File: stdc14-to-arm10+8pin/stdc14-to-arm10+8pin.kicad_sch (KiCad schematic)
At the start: 3 parts, among them J1 Conn_ARM_JTAG_SWD_10, J2 Conn_ST_STDC14, J3 Conn_02x04_Counter_Clockwise

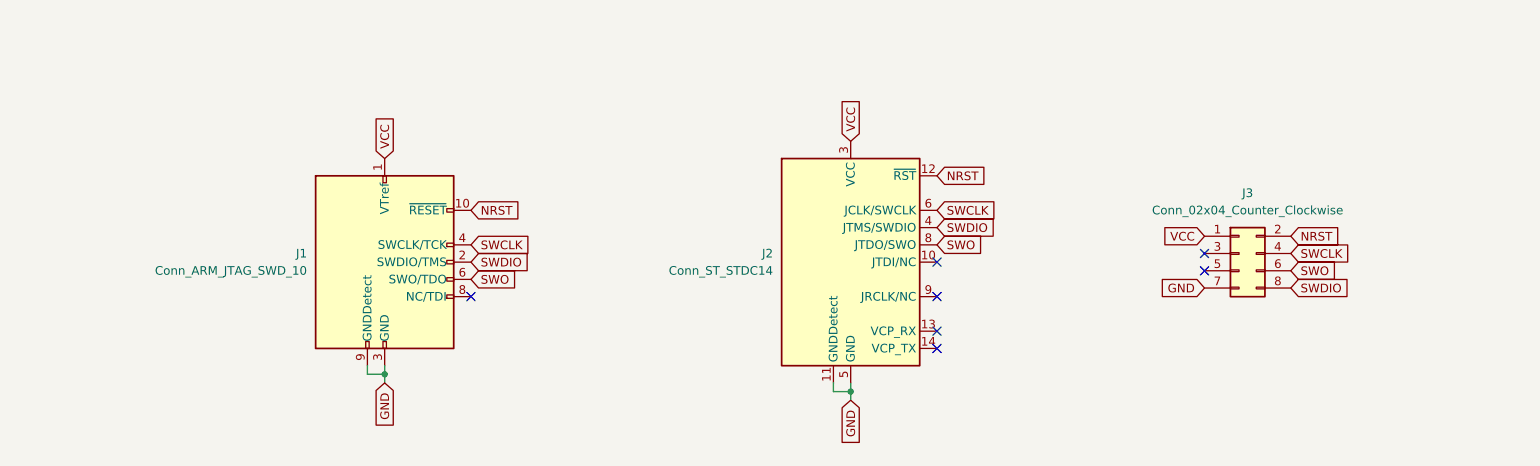
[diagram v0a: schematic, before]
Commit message: prob fin?
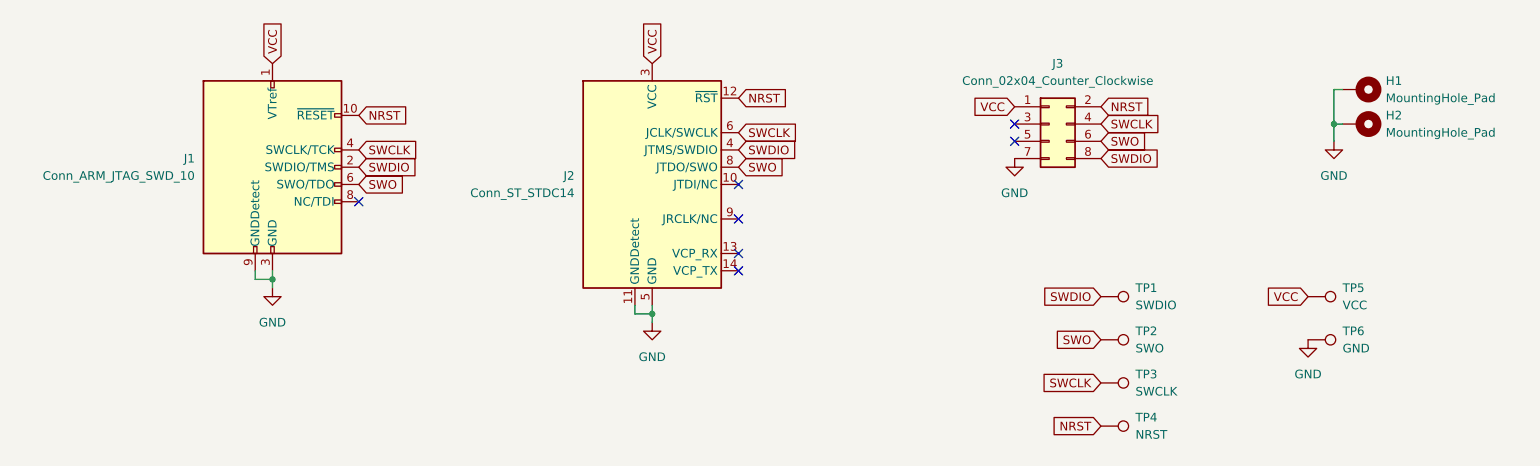
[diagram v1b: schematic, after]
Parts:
- added H1, H2: MountingHole_Pad, MountingHole:MountingHole_2.7mm_M2.5_Pad, symbol Mechanical:MountingHole_Pad
- added TP1: SWDIO, TestPoint:TestPoint_Pad_D1.0mm, symbol Connector:TestPoint
- added TP2: SWO, TestPoint:TestPoint_Pad_D1.0mm, symbol Connector:TestPoint
- added TP3: SWCLK, TestPoint:TestPoint_Pad_D1.0mm, symbol Connector:TestPoint
- added TP4: NRST, TestPoint:TestPoint_Pad_D1.0mm, symbol Connector:TestPoint
- added TP5: VCC, TestPoint:TestPoint_Pad_D1.0mm, symbol Connector:TestPoint
- added TP6: GND, TestPoint:TestPoint_Pad_D1.0mm, symbol Connector:TestPoint
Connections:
- net GND: now also H1.1, H2.1, TP6.1
- net NRST: now also TP4.1
- net SWCLK: now also TP3.1
- net SWDIO: now also TP1.1
- net SWO: now also TP2.1
- net VCC: now also TP5.1
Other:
- moved on the sheet: J1, J2, J3
